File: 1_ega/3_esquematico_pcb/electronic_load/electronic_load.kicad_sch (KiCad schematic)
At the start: 39 parts, among them J1 Encoder, J10 5V, J11 LOAD, J12 FAN, J13 RTC_I2C, J14 INA219, J15 EGB_I2C, J16 EGB_UART, J2 LCD_I2C, J3 GND, J4 MOS_GATE, J5 MOS_PWM, J6 Vload_LPF, J7 GND, J8 MOS_LPF, J9 TEMP_DIODE, Q1 IRF540N, Q2 2n2222, Q3 BC327, Q4 BC327, SW1 BTN_MENU, SW2 BTN_STOP, U1 LM358

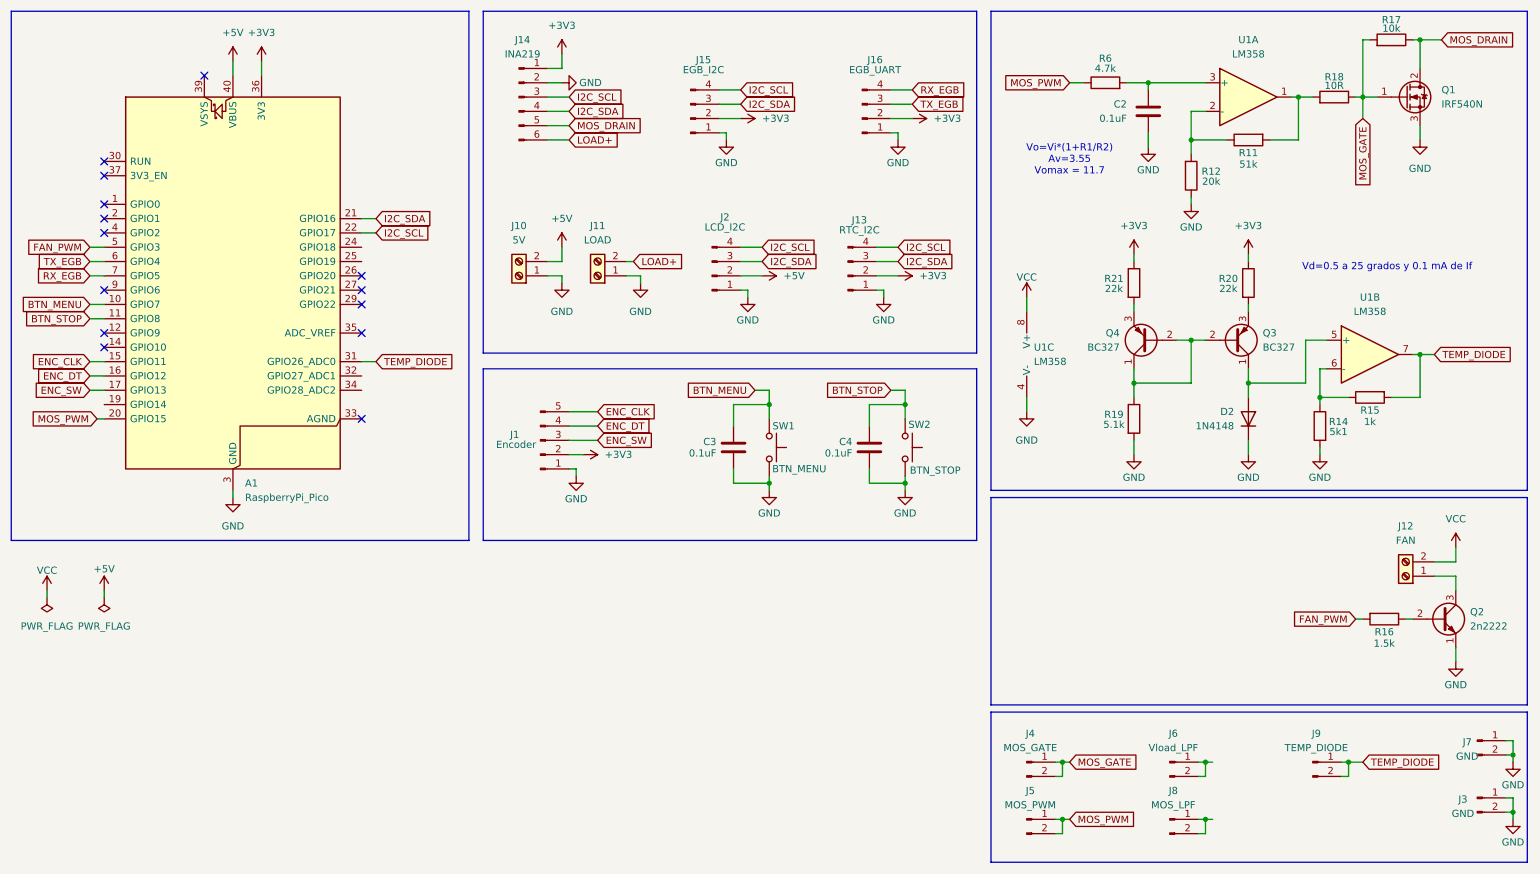
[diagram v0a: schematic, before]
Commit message: feat: schematic and pcb full v1
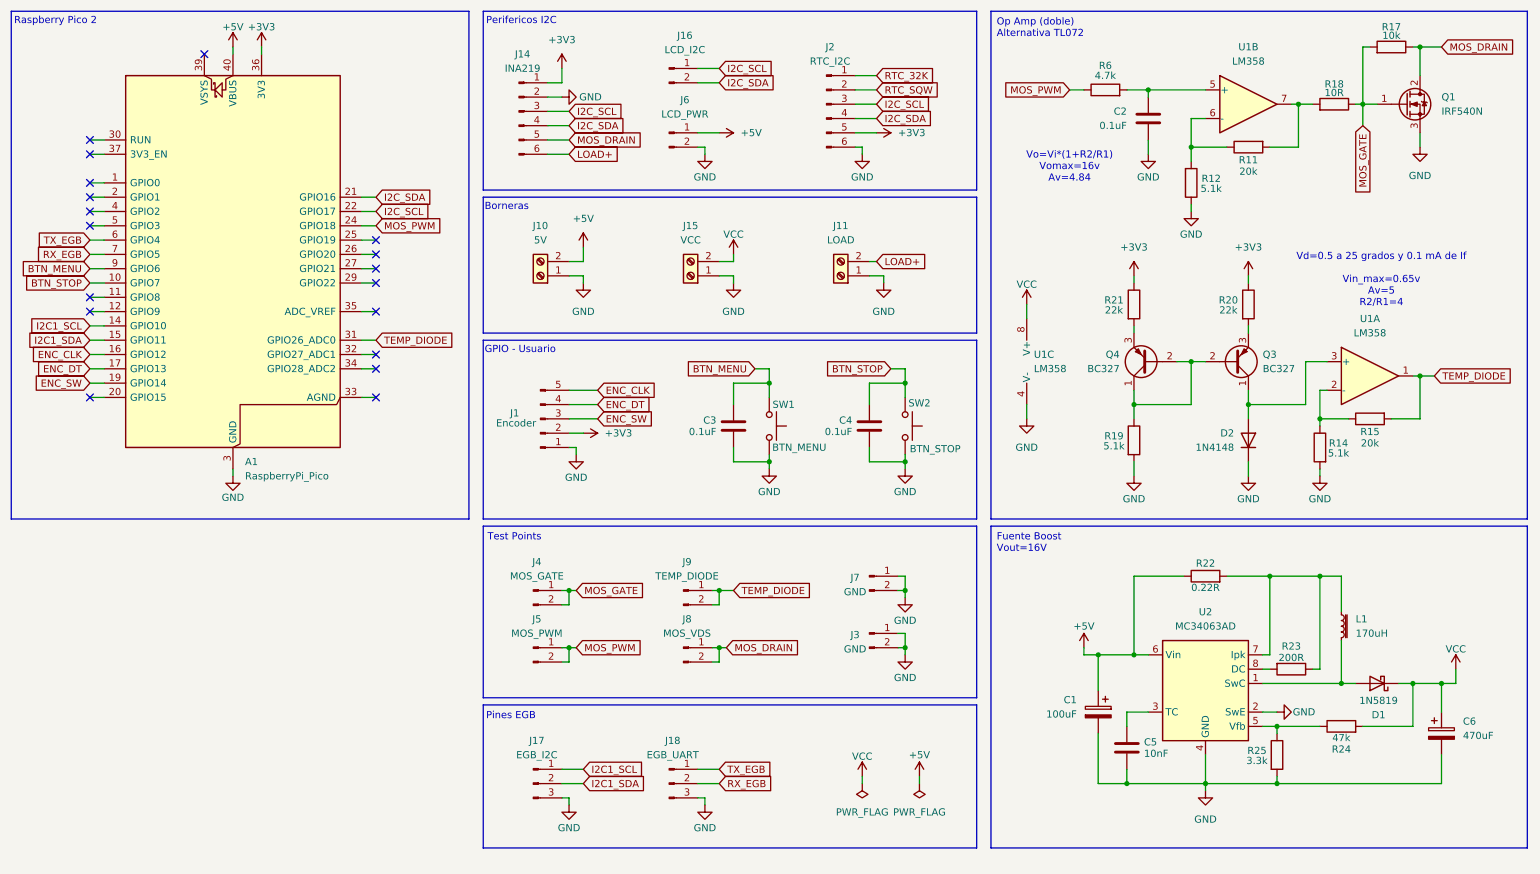
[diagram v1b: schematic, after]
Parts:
- removed J12: FAN, TerminalBlock_Phoenix:TerminalBlock_Phoenix_MKDS-1,5-2-5.08_1x02_P5.08mm_Horizontal, symbol Connector:Screw_Terminal_01x02
- removed J13: RTC_I2C, Connector_PinSocket_2.54mm:PinSocket_1x04_P2.54mm_Vertical, symbol Connector:Conn_01x04_Pin
- removed J15: EGB_I2C, Connector_PinSocket_2.54mm:PinSocket_1x04_P2.54mm_Vertical, symbol Connector:Conn_01x04_Pin
- removed J16: EGB_UART, Connector_PinSocket_2.54mm:PinSocket_1x04_P2.54mm_Vertical, symbol Connector:Conn_01x04_Pin
- removed J2: LCD_I2C, Connector_PinSocket_2.54mm:PinSocket_1x04_P2.54mm_Vertical, symbol Connector:Conn_01x04_Pin
- removed Q2: 2n2222, Package_TO_SOT_THT:TO-92L_Inline_Wide, symbol Transistor_BJT:2N2219
- removed R16: 1.5k, Resistor_THT:R_Axial_DIN0207_L6.3mm_D2.5mm_P10.16mm_Horizontal, symbol Device:R
- added C1: 100uF, Capacitor_THT:CP_Radial_D6.3mm_P2.50mm, symbol Device:C_Polarized
- added C5: 10nF, Capacitor_THT:C_Disc_D3.4mm_W2.1mm_P2.50mm, symbol Device:C
- added C6: 470uF, Capacitor_THT:CP_Radial_D6.3mm_P2.50mm, symbol Device:C_Polarized
- added D1: 1N5819, Diode_THT:D_DO-41_SOD81_P10.16mm_Horizontal, symbol Diode:1N5819
- added J15: VCC, TerminalBlock_Phoenix:TerminalBlock_Phoenix_MKDS-1,5-2-5.08_1x02_P5.08mm_Horizontal, symbol Connector:Screw_Terminal_01x02
- added J16: LCD_I2C, Connector_PinHeader_2.54mm:PinHeader_1x02_P2.54mm_Vertical, symbol Connector:Conn_01x02_Pin
- added J17: EGB_I2C, Connector_PinSocket_2.54mm:PinSocket_1x03_P2.54mm_Vertical, symbol Connector:Conn_01x03_Pin
- added J18: EGB_UART, Connector_PinSocket_2.54mm:PinSocket_1x03_P2.54mm_Vertical, symbol Connector:Conn_01x03_Pin
- added J2: RTC_I2C, Connector_PinSocket_2.54mm:PinSocket_1x06_P2.54mm_Vertical, symbol Connector:Conn_01x06_Pin
- added L1: 170uH, Inductor_THT:L_Radial_D10.5mm_P5.00mm_Abacron_AISR-01, symbol Device:L_Iron_Small
- added R22: 0.22R, Resistor_THT:R_Axial_DIN0207_L6.3mm_D2.5mm_P10.16mm_Horizontal, symbol Device:R
- added R23: 200R, Resistor_THT:R_Axial_DIN0207_L6.3mm_D2.5mm_P10.16mm_Horizontal, symbol Device:R
- added R24: 47k, Resistor_THT:R_Axial_DIN0207_L6.3mm_D2.5mm_P10.16mm_Horizontal, symbol Device:R
- added R25: 3.3k, Resistor_THT:R_Axial_DIN0207_L6.3mm_D2.5mm_P10.16mm_Horizontal, symbol Device:R
- added U2: MC34063AD, Package_SO:SOIC-8_3.9x4.9mm_P1.27mm, symbol Regulator_Switching:MC34063AD
- A1: footprint Module:RaspberryPi_Pico_Common_THT -> electronic_load:RaspberryPi_Pico_2_THT
- J1: footprint Connector_PinSocket_2.54mm:PinSocket_1x05_P2.54mm_Vertical -> Connector_PinHeader_2.54mm:PinHeader_1x05_P2.54mm_Vertical
- J14: footprint Connector_PinSocket_2.54mm:PinSocket_1x06_P2.54mm_Vertical -> electronic_load:INA219
- J3, J4, J5, J7, J9: footprint Connector_PinSocket_2.54mm:PinSocket_1x02_P2.54mm_Vertical -> Connector_PinHeader_2.54mm:PinHeader_1x02_P2.54mm_Vertical
- J6: value Vload_LPF -> LCD_PWR; footprint Connector_PinSocket_2.54mm:PinSocket_1x02_P2.54mm_Vertical -> Connector_PinHeader_2.54mm:PinHeader_1x02_P2.54mm_Vertical
- J8: value MOS_LPF -> MOS_VDS; footprint Connector_PinSocket_2.54mm:PinSocket_1x02_P2.54mm_Vertical -> Connector_PinHeader_2.54mm:PinHeader_1x02_P2.54mm_Vertical
- R11: value 51k -> 20k
- R12: value 20k -> 5.1k
- R14: value 5k1 -> 5.1k
- R15: value 1k -> 20k
- SW1, SW2: footprint Button_Switch_THT:SW_PUSH_6mm -> Connector_PinHeader_2.54mm:PinHeader_1x02_P2.54mm_Vertical
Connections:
- net +3V3: now also J2.5 (Pin_5)
- net +5V: now also J6.1 (Pin_1), C1.1, R22.1, U2.6 (Vin)
- net BTN_MENU: now also A1.9 (GPIO6); no longer A1.10 (GPIO7)
- net BTN_STOP: now also A1.10 (GPIO7); no longer A1.11 (GPIO8)
- net ENC_CLK: now also A1.16 (GPIO12); no longer A1.15 (GPIO11)
- net ENC_DT: now also A1.17 (GPIO13); no longer A1.16 (GPIO12)
- net ENC_SW: now also A1.19 (GPIO14); no longer A1.17 (GPIO13)
- net GND: now also J6.2 (Pin_2), C1.2, C5.1, C6.2, J15.1 (Pin_1), J17.3 (Pin_3), J18.3 (Pin_3), J2.6 (Pin_6), R25.2, U2.2 (SwE), U2.4 (GND)
- net I2C_SCL: now also J16.1 (Pin_1), J2.3 (Pin_3)
- net I2C_SDA: now also J16.2 (Pin_2), J2.4 (Pin_4)
- net MOS_DRAIN: now also J8.1 (Pin_1), J8.2 (Pin_2)
- net MOS_PWM: now also A1.24 (GPIO18); no longer A1.20 (GPIO15)
- net RX_EGB: now also J18.2 (Pin_2)
- net TEMP_DIODE: now also U1.1; no longer U1.7
- net TX_EGB: now also J18.1 (Pin_1)
- net VCC: now also C6.1, D1.1 (K), J15.2 (Pin_2), R24.2
- net at C2.1, R6.2: now also U1.5 (+); no longer U1.3 (+)
- net at R11.1, R12.2: now also U1.6 (-); no longer U1.2 (-)
- net at R11.2, R18.2: now also U1.7; no longer U1.1
- net at R14.1, R15.1: now also U1.2 (-); no longer U1.6 (-)
- net at D2.2 (A), Q3.1 (C): now also U1.3 (+); no longer U1.5 (+)
- net I2C1_SCL: now reaches A1.14 (GPIO10)
- net I2C1_SCL: now also J17.1 (Pin_1)
- net FAN_PWM: no longer names the net of A1.5 (GPIO3)
- new net: L1.1, R22.2, R23.1, U2.7 (Ipk)
- new net: D1.2 (A), L1.2, U2.1 (SwC)
- new net: R24.1, R25.1, U2.5 (Vfb)
- new net: C5.2, U2.3 (TC)
- new net: R23.2, U2.8 (DC)
- new net I2C1_SDA: A1.15 (GPIO11), J17.2 (Pin_2)
- new net RTC_32K: J2.1 (Pin_1)
- new net RTC_SQW: J2.2 (Pin_2)
- no-connect marks 14 -> 18
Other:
- note added: "Borneras"
- note added: "Fuente Boost Vout=16V"
- note added: "GPIO - Usuario"
- note added: "Op Amp (doble) Alternativa TL072"
- note added: "Perifericos I2C"
- note added: "Pines EGB"
- note added: "Raspberry Pico 2"
- note added: "Test Points"
- note added: "Vd=0.5 a 25 grados y 0.1 mA de If Vin_max=0.65v Av=5 R2/R1=4"
- note added: "Vo=Vi*(1+R2/R1) Vomax=16v Av=4.84"
- note removed: "Vd=0.5 a 25 grados y 0.1 mA de If"
- note removed: "Vo=Vi*(1+R1/R2) Av=3.55 Vomax = 11.7"
- moved on the sheet: A1, C2, C3, C4, D2, J1, J10, J11, J14, J3, J4, J5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
